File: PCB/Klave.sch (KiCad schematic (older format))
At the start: 19 parts

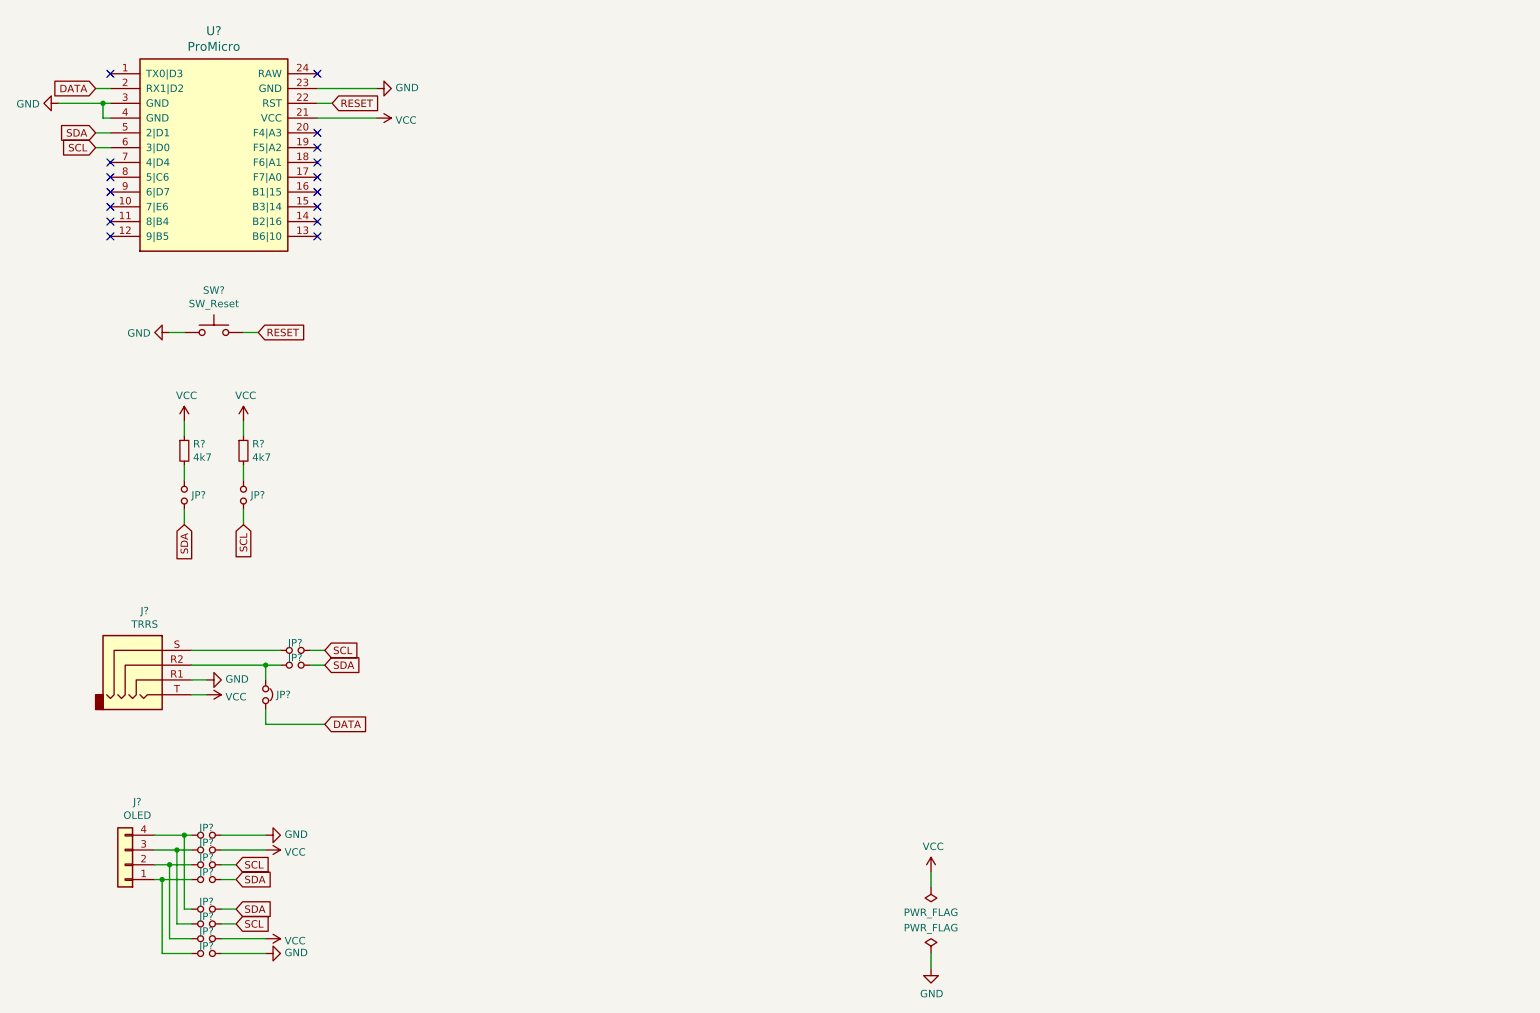
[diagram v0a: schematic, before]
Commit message: Add key matrix
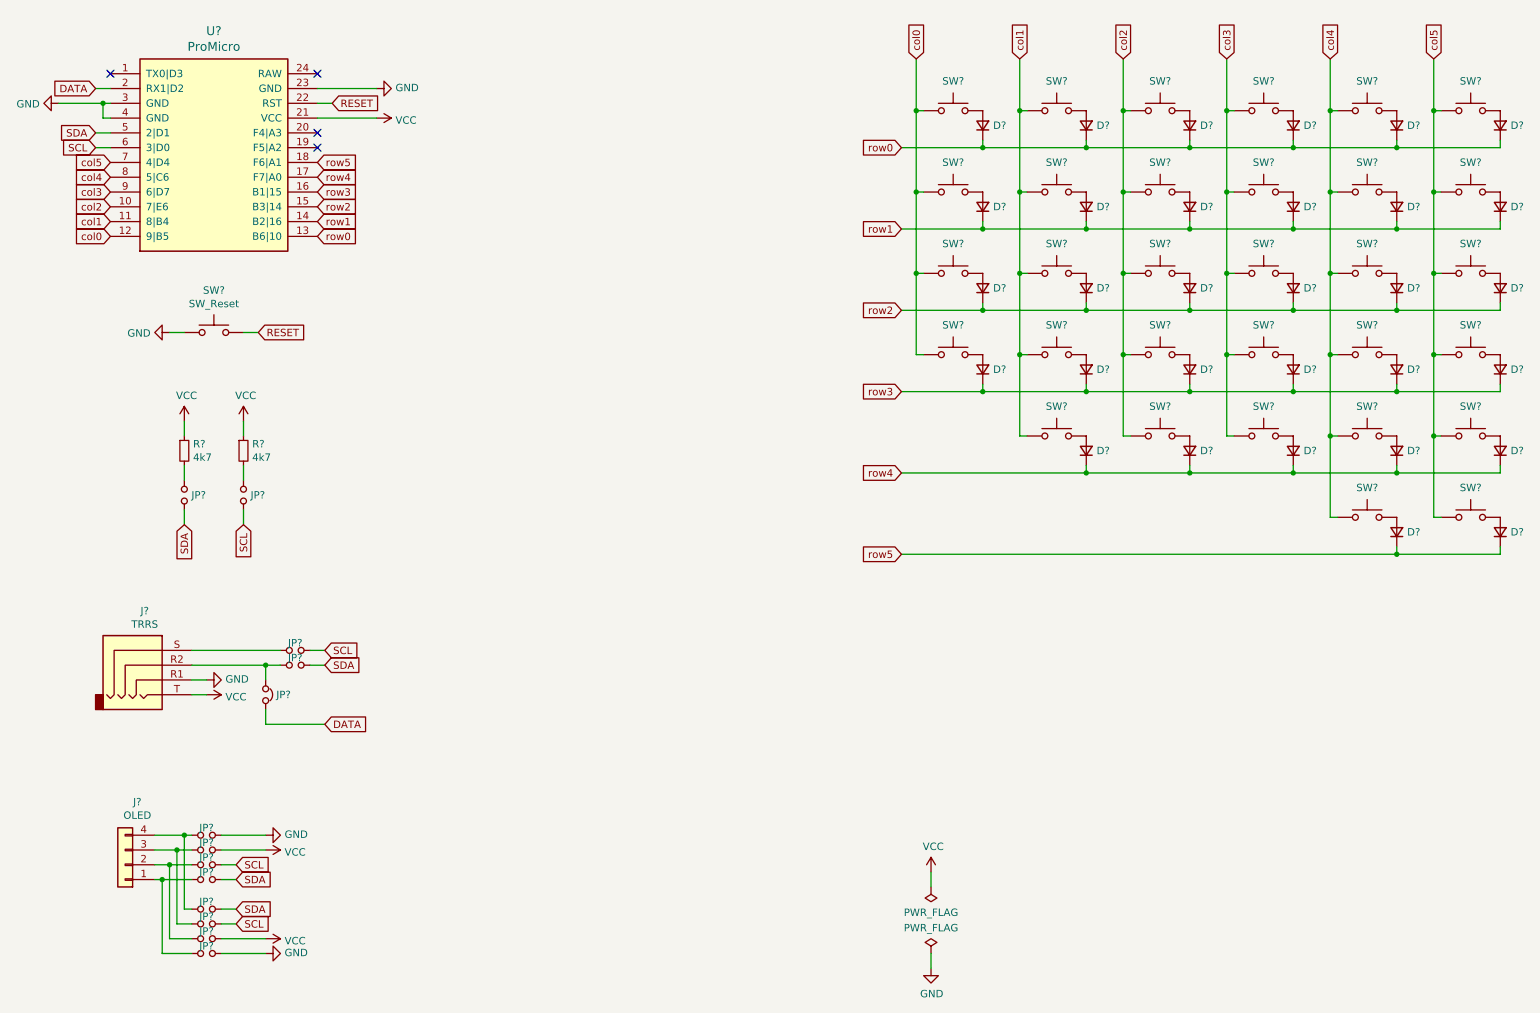
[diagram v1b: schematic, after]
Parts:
- added D? (x31): D_Small, symbol Device:D_Small
- added SW? (x31): SW_Key, symbol Switch:SW_Push
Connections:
- net col2: now reaches U?.10 (7|E6)
- net col2: now also SW?.1, SW?.1, SW?.1, SW?.1, SW?.1
- net col1: now reaches U?.11 (8|B4)
- net col1: now also SW?.1, SW?.1, SW?.1, SW?.1, SW?.1
- net col0: now reaches U?.12 (9|B5)
- net col0: now also SW?.1, SW?.1, SW?.1, SW?.1
- net row0: now reaches U?.13 (B6|10)
- net row0: now also D?.1 (K), D?.1 (K), D?.1 (K), D?.1 (K), D?.1 (K), D?.1 (K)
- net row1: now reaches U?.14 (B2|16)
- net row1: now also D?.1 (K), D?.1 (K), D?.1 (K), D?.1 (K), D?.1 (K), D?.1 (K)
- net row2: now reaches U?.15 (B3|14)
- net row2: now also D?.1 (K), D?.1 (K), D?.1 (K), D?.1 (K), D?.1 (K), D?.1 (K)
- net row3: now reaches U?.16 (B1|15)
- net row3: now also D?.1 (K), D?.1 (K), D?.1 (K), D?.1 (K), D?.1 (K), D?.1 (K)
- net row4: now reaches U?.17 (F7|A0)
- net row4: now also D?.1 (K), D?.1 (K), D?.1 (K), D?.1 (K), D?.1 (K)
- net row5: now reaches U?.18 (F6|A1)
- net row5: now also D?.1 (K), D?.1 (K)
- net col5: now reaches U?.7 (4|D4)
- net col5: now also SW?.1, SW?.1, SW?.1, SW?.1, SW?.1, SW?.1
- net col4: now reaches U?.8 (5|C6)
- net col4: now also SW?.1, SW?.1, SW?.1, SW?.1, SW?.1, SW?.1
- net col3: now reaches U?.9 (6|D7)
- net col3: now also SW?.1, SW?.1, SW?.1, SW?.1, SW?.1
- new net: D?.2 (A), SW?.2 (x31)
- no-connect marks 16 -> 4
